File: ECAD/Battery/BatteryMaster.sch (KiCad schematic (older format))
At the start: 87 parts, among them J1 BOOT, J2 SWD, Q1 Si4186DY, Q10 Si4186DY, Q11 IRF7458, Q12 Si4186DY, Q2 IRF7458, Q3 IRF7458, Q4 Si4186DY, Q5 2N7002, Q6 IRF7425, Q7 IRF7458, Q8 IRF7458, Q9 IRF7458, SW1 INHIBIT4, SW2 INHIBIT5, SW3 INHIBIT6, U1 LM1117-3.3, U2 INA181A2, U3 BQ29209, U4 LM358, U5 MAX6369, U6 LTC4365TS8-1, U7 STM32F103C8Tx, Y1 8MHz

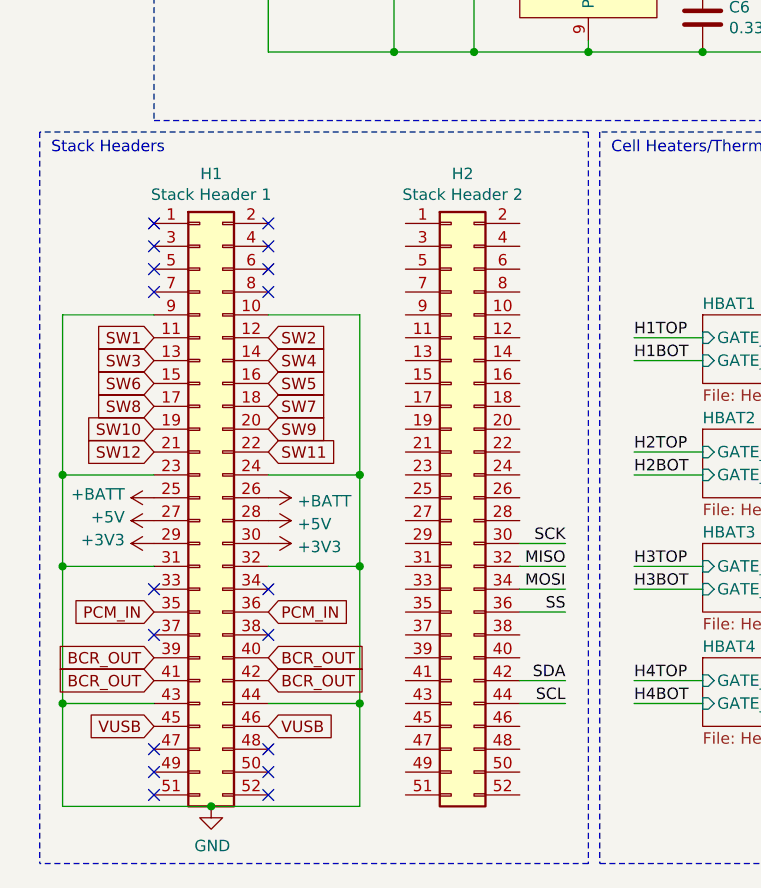
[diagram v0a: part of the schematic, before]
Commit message: Restandardize stack headers a bit
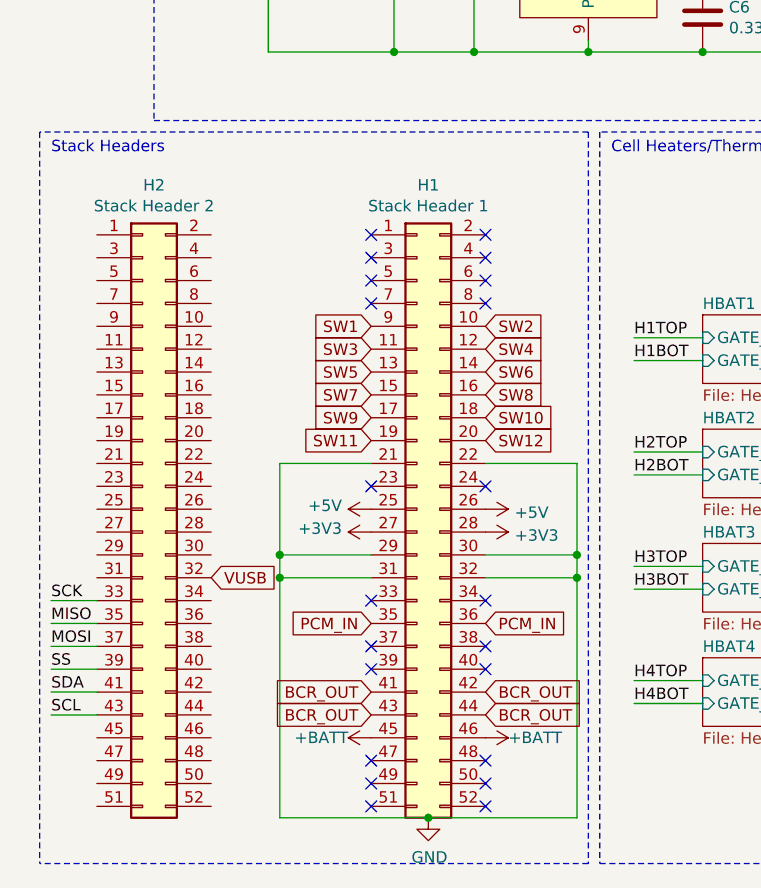
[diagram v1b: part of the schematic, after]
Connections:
- net +3V3: now also H1.27 (Pin_27), H1.28 (Pin_28); no longer H1.29 (Pin_29), H1.30 (Pin_30)
- net +5V: now also H1.25 (Pin_25), H1.26 (Pin_26); no longer H1.27 (Pin_27), H1.28 (Pin_28)
- net +BATT: now also H1.45 (Pin_45), H1.46 (Pin_46); no longer H1.25 (Pin_25), H1.26 (Pin_26)
- net BCR_OUT: now also H1.43 (Pin_43), H1.44 (Pin_44); no longer H1.39 (Pin_39), H1.40 (Pin_40)
- net GND: now also H1.21 (Pin_21), H1.22 (Pin_22), H1.29 (Pin_29), H1.30 (Pin_30); no longer H1.10 (Pin_10), H1.23 (Pin_23), H1.24 (Pin_24), H1.43 (Pin_43), H1.44 (Pin_44), H1.9 (Pin_9)
- net MISO: now also H2.35 (Pin_35); no longer H2.32 (Pin_32)
- net MOSI: now also H2.37 (Pin_37); no longer H2.34 (Pin_34)
- net SCK: now also H2.33 (Pin_33); no longer H2.30 (Pin_30)
- net SCL: now also H2.43 (Pin_43); no longer H2.44 (Pin_44)
- net SDA: now also H2.41 (Pin_41); no longer H2.42 (Pin_42)
- net SS: now also H2.39 (Pin_39); no longer H2.36 (Pin_36)
- net SW1: now also H1.9 (Pin_9); no longer H1.11 (Pin_11)
- net SW10: now also H1.18 (Pin_18); no longer H1.19 (Pin_19)
- net SW11: now also H1.19 (Pin_19); no longer H1.22 (Pin_22)
- net SW12: now also H1.20 (Pin_20); no longer H1.21 (Pin_21)
- net SW2: now also H1.10 (Pin_10); no longer H1.12 (Pin_12)
- net SW3: now also H1.11 (Pin_11); no longer H1.13 (Pin_13)
- net SW4: now also H1.12 (Pin_12); no longer H1.14 (Pin_14)
- net SW5: now also H1.13 (Pin_13); no longer H1.16 (Pin_16)
- net SW6: now also H1.14 (Pin_14); no longer H1.15 (Pin_15)
- net SW7: now also H1.15 (Pin_15); no longer H1.18 (Pin_18)
- net SW8: now also H1.16 (Pin_16); no longer H1.17 (Pin_17)
- net SW9: now also H1.17 (Pin_17); no longer H1.20 (Pin_20)
- net VUSB: now also H2.32 (Pin_32); no longer H1.45 (Pin_45), H1.46 (Pin_46)
- no-connect marks 19 -> 23
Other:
- moved on the sheet: H1, H2
